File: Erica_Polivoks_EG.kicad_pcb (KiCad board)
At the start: 2 copper layers, 40.3 x 106 mm, 92 parts, among them J1 GATE IN, J2 INV EG OUT, J3 Eurorack_Power_10pin_Unshroud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, J4 GATE DELAY OUT, J5 EG OUT, Q1 2N3904, Q2 2N3904, Q3 2N3904, Q4 2N3904, Q5 2N3904, Q6 2N3904, Q7 2N3906, Q8 2N3906, Q9 2N3906, SW1 SW_DPDT_x2, U1 TL074

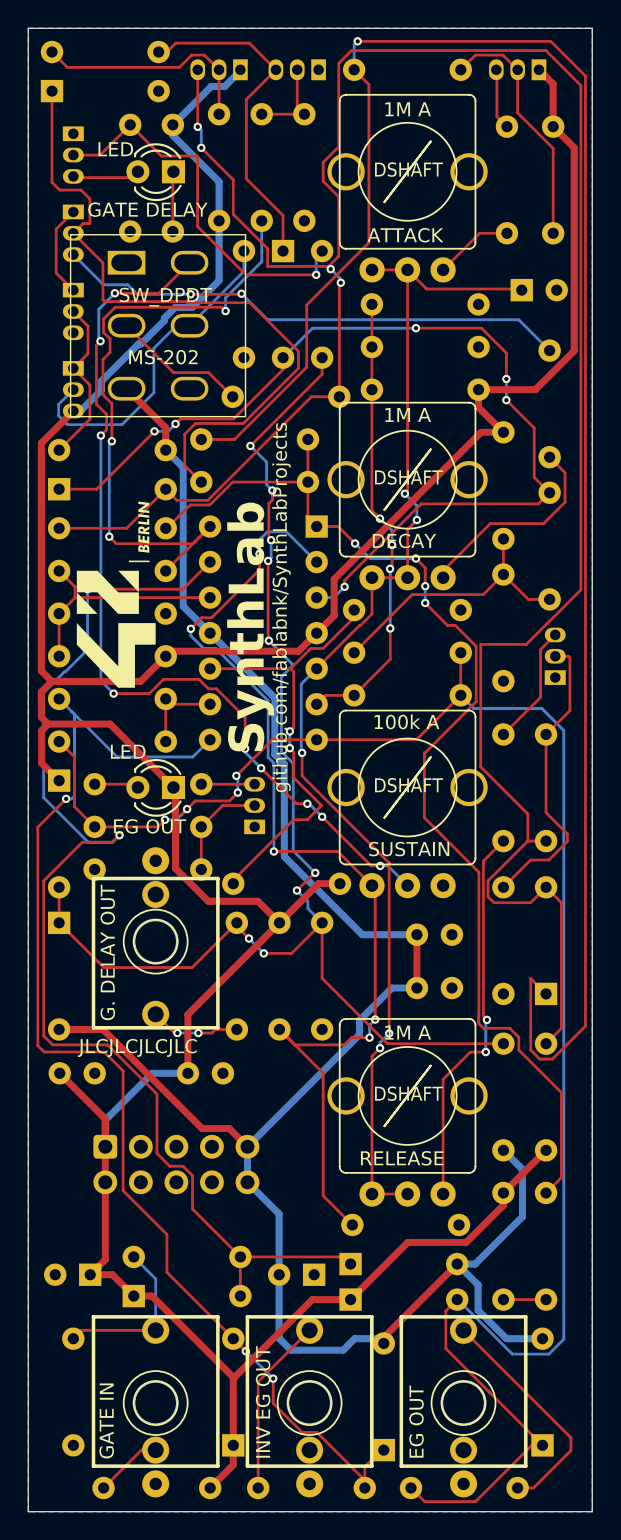
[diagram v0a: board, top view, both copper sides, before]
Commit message: v1.1 ready for final check
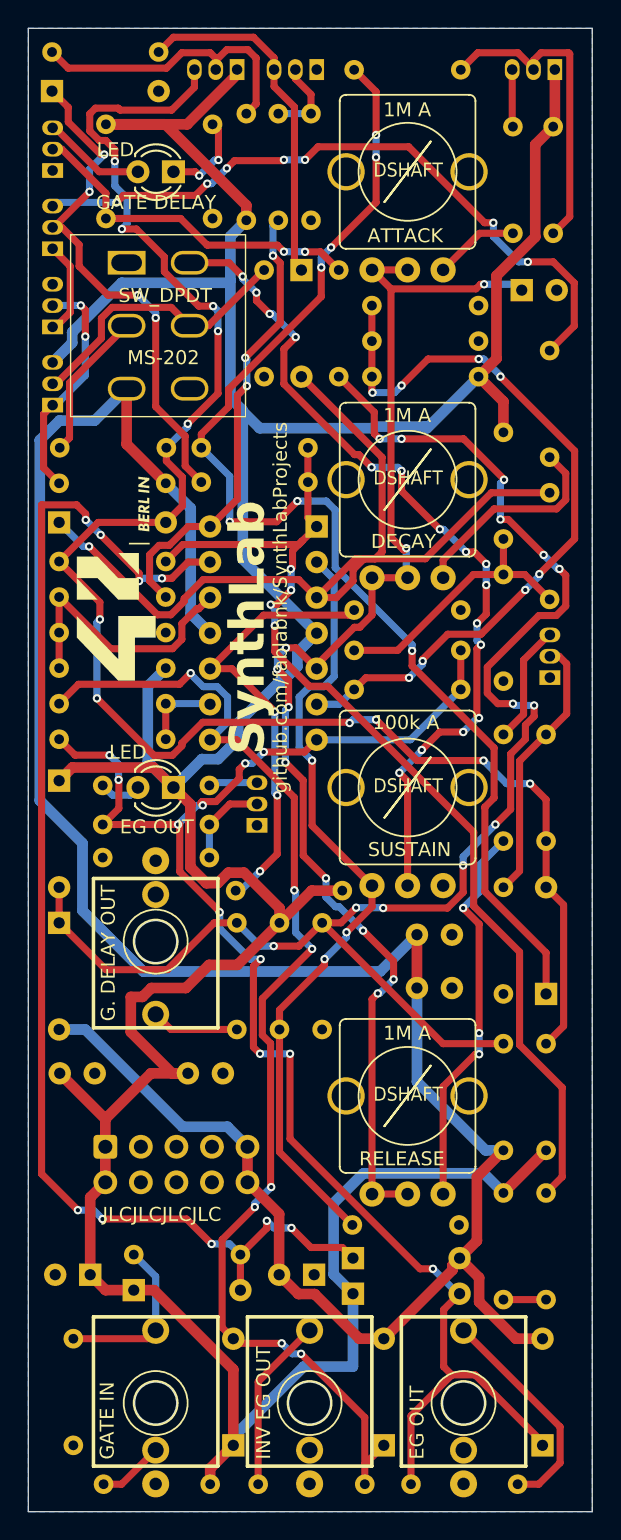
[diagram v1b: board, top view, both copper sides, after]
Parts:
- R1, R10, R11, R12, R13, R14, R15, R16, R17, R18, R19, R2, R20, R21, R22, R23, R24, R25, R26, R27, R28, R29, R3, R30, R31, R32, R33, R35, R36, R37, R38, R39, R4, R40, R41, R42, R43, R44, R45, R46, R47, R48, R49, R5, R50, R51, R6, R7, R8, R9: footprint Resistor_THT:R_Axial_DIN0207_L6.3mm_D2.5mm_P7.62mm_Horizontal -> Library:R_Axial_DIN0204_L3.6mm_D1.6mm_P7.62mm_Horizontal_Widened
- R34: value NU 39K -> NU 39k; footprint Resistor_THT:R_Axial_DIN0207_L6.3mm_D2.5mm_P7.62mm_Horizontal -> Library:R_Axial_DIN0204_L3.6mm_D1.6mm_P7.62mm_Horizontal_Widened
- moved R19 12.9 mm to (60.8, 80.8)
- moved R38 6.91 mm to (56.5, 64.4), turned to 0 degrees
- moved R40 4.78 mm to (56.5, 57.7), turned to 0 degrees
- moved Q9 2.58 mm to (52.7, 71.9), turned to 90 degrees
- moved Q4 2.58 mm to (52.7, 60.7), turned to 90 degrees
- moved Q3 2.58 mm to (52.7, 66.3), turned to 90 degrees
- moved Q6 2.58 mm to (52.7, 77.5), turned to 90 degrees
- moved D5 2.37 mm to (53.2, 86.1)
- moved R20 2.37 mm to (53.2, 88.9)
- moved R26 2.37 mm to (53.2, 83.3)
- moved R25 1.98 mm to (67.8, 75.7)
- moved R13 1.95 mm to (66.5, 64.5)
- moved D3 1.89 mm to (70.5, 68.1)
- moved R7 1.86 mm to (53.2, 91.4)
- moved R39 1.80 mm to (73.2, 68.1)
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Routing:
- net Net-(D4-A): track 173.0 -> 122.6 mm, vias 4 -> 11
- net Net-(D4-K): track 132.4 -> 88.8 mm, vias 1 -> 7
- net -12V: track 139.4 -> 170.8 mm
- net +12V: track 259.6 -> 284.0 mm
- net Net-(U1B--): track 32.6 -> 54.3 mm, vias 4 -> 8
- net Net-(U1A--): track 75.3 -> 56.6 mm, vias 5 -> 3
- net Net-(D12-K): track 91.6 -> 108.7 mm, vias 9 -> 13
- net Net-(D14-K): track 128.8 -> 111.9 mm, vias 4 -> 11
- net Net-(R10-Pad2): track 45.4 -> 33.1 mm
- net Net-(Q3-C): track 36.9 -> 49.2 mm, vias 2 -> 7
- net Net-(D6-K): track 49.3 -> 37.3 mm, vias 0 -> 4
- net Net-(U1B-+): track 88.4 -> 95.6 mm, vias 5 -> 10
- net Net-(D1-K): track 85.9 -> 92.8 mm, vias 2 -> 9
- net Net-(Q7-B): track 16.4 -> 22.0 mm
- net Net-(Q8-B): track 17.7 -> 23.1 mm
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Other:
- board text removed: "▲"
- board text removed: "▶"
